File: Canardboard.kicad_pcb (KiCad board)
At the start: 4 copper layers, 50 x 58.8 mm, 149 parts, among them IC1 SIC437DED-T1-GE3, J1 RBUS, J2 USB_C_Receptacle_USB2.0, J3 Micro_SD_Card_Det, J4 Conn_01x02_Male, J5 Conn_01x03_Male, J6 Conn_01x03_Male, J7 Conn_01x03_Male, Q1 PXP012-30QLJ, Q2 PXP012-30QLJ, Q4 PXP012-30QLJ, Q6 PXP012-30QLJ, U1 ESP32-S3, U10 MP28167GQ-A-Z, U2 SN65HVD230, U3 LTC4412xS6, U4 LTC4412xS6, U7 ICM-20608-G, U8 MMC5983MA, Y1 40MHz±10ppm

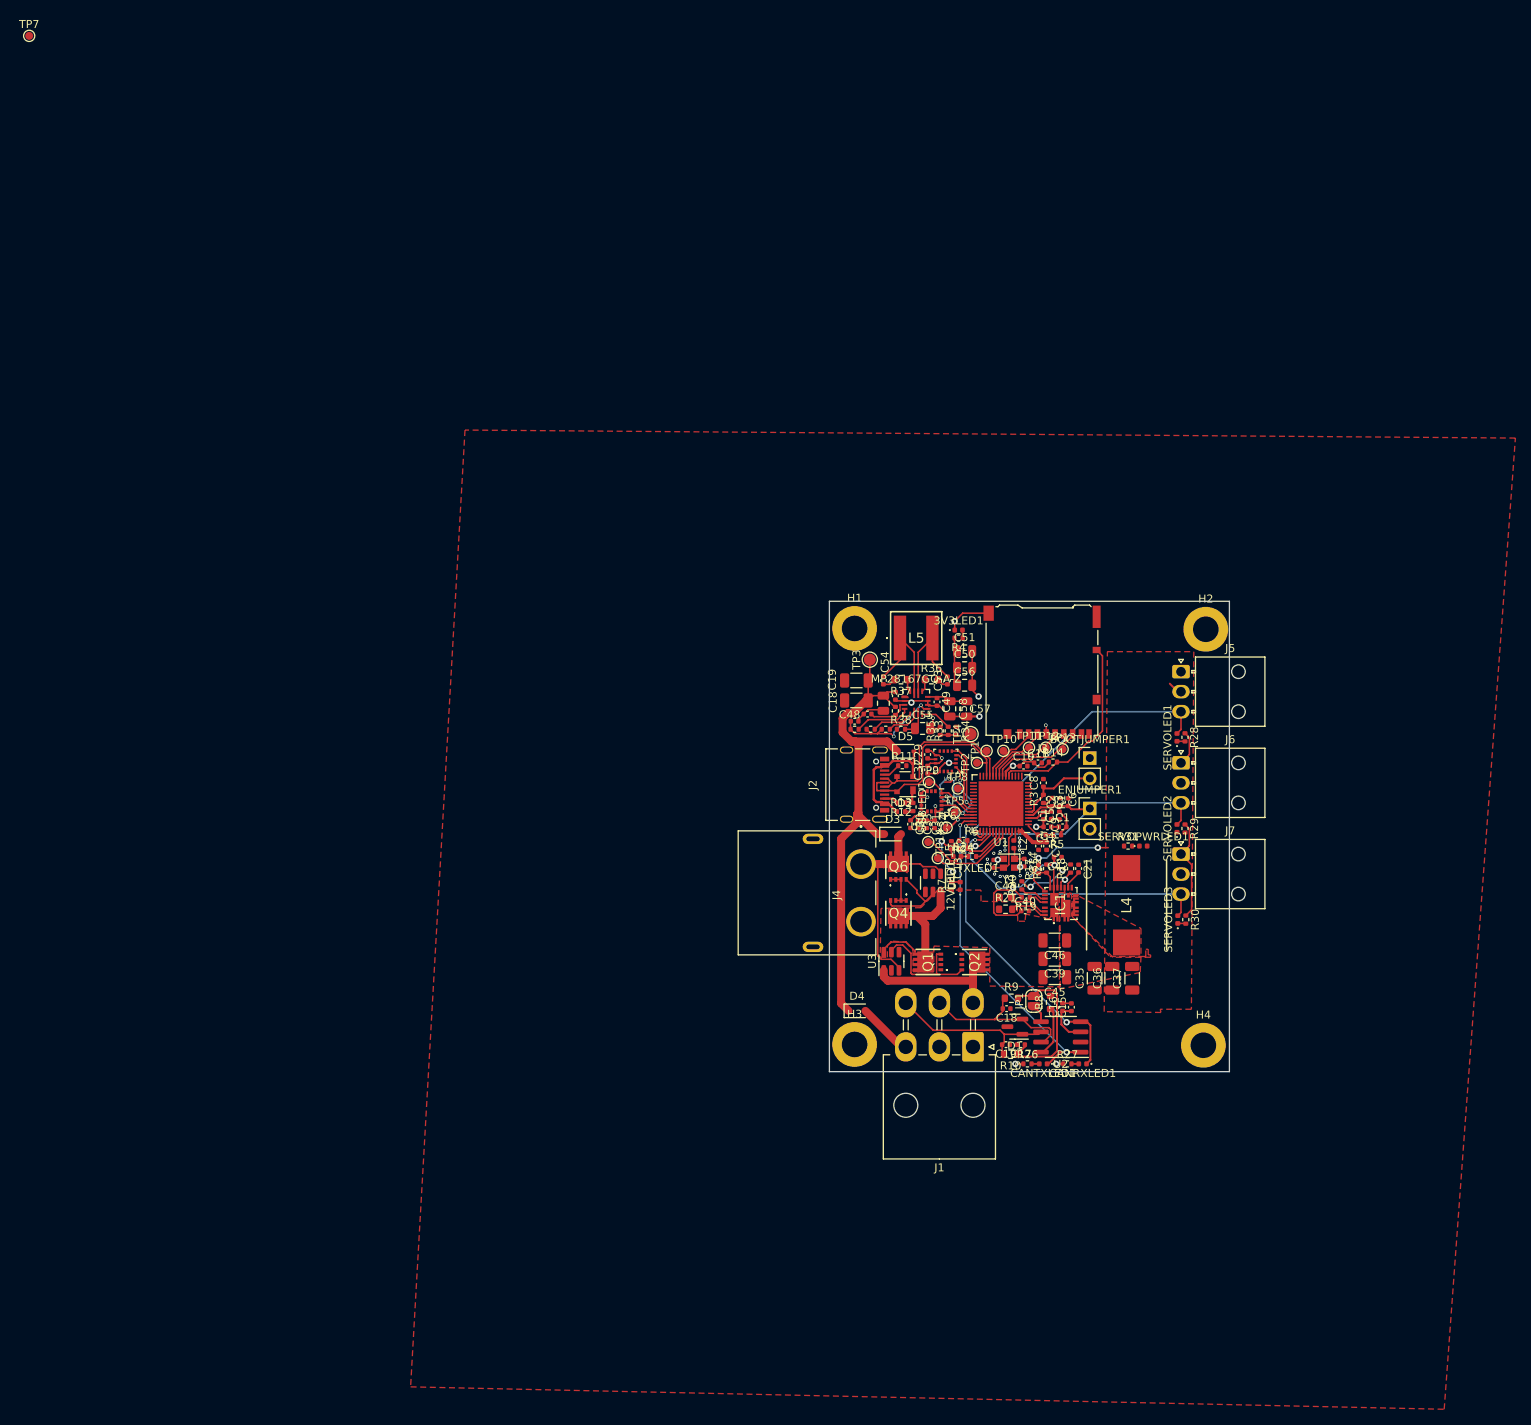
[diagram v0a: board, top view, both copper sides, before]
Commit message: weird 3v3 and 3.3v bug
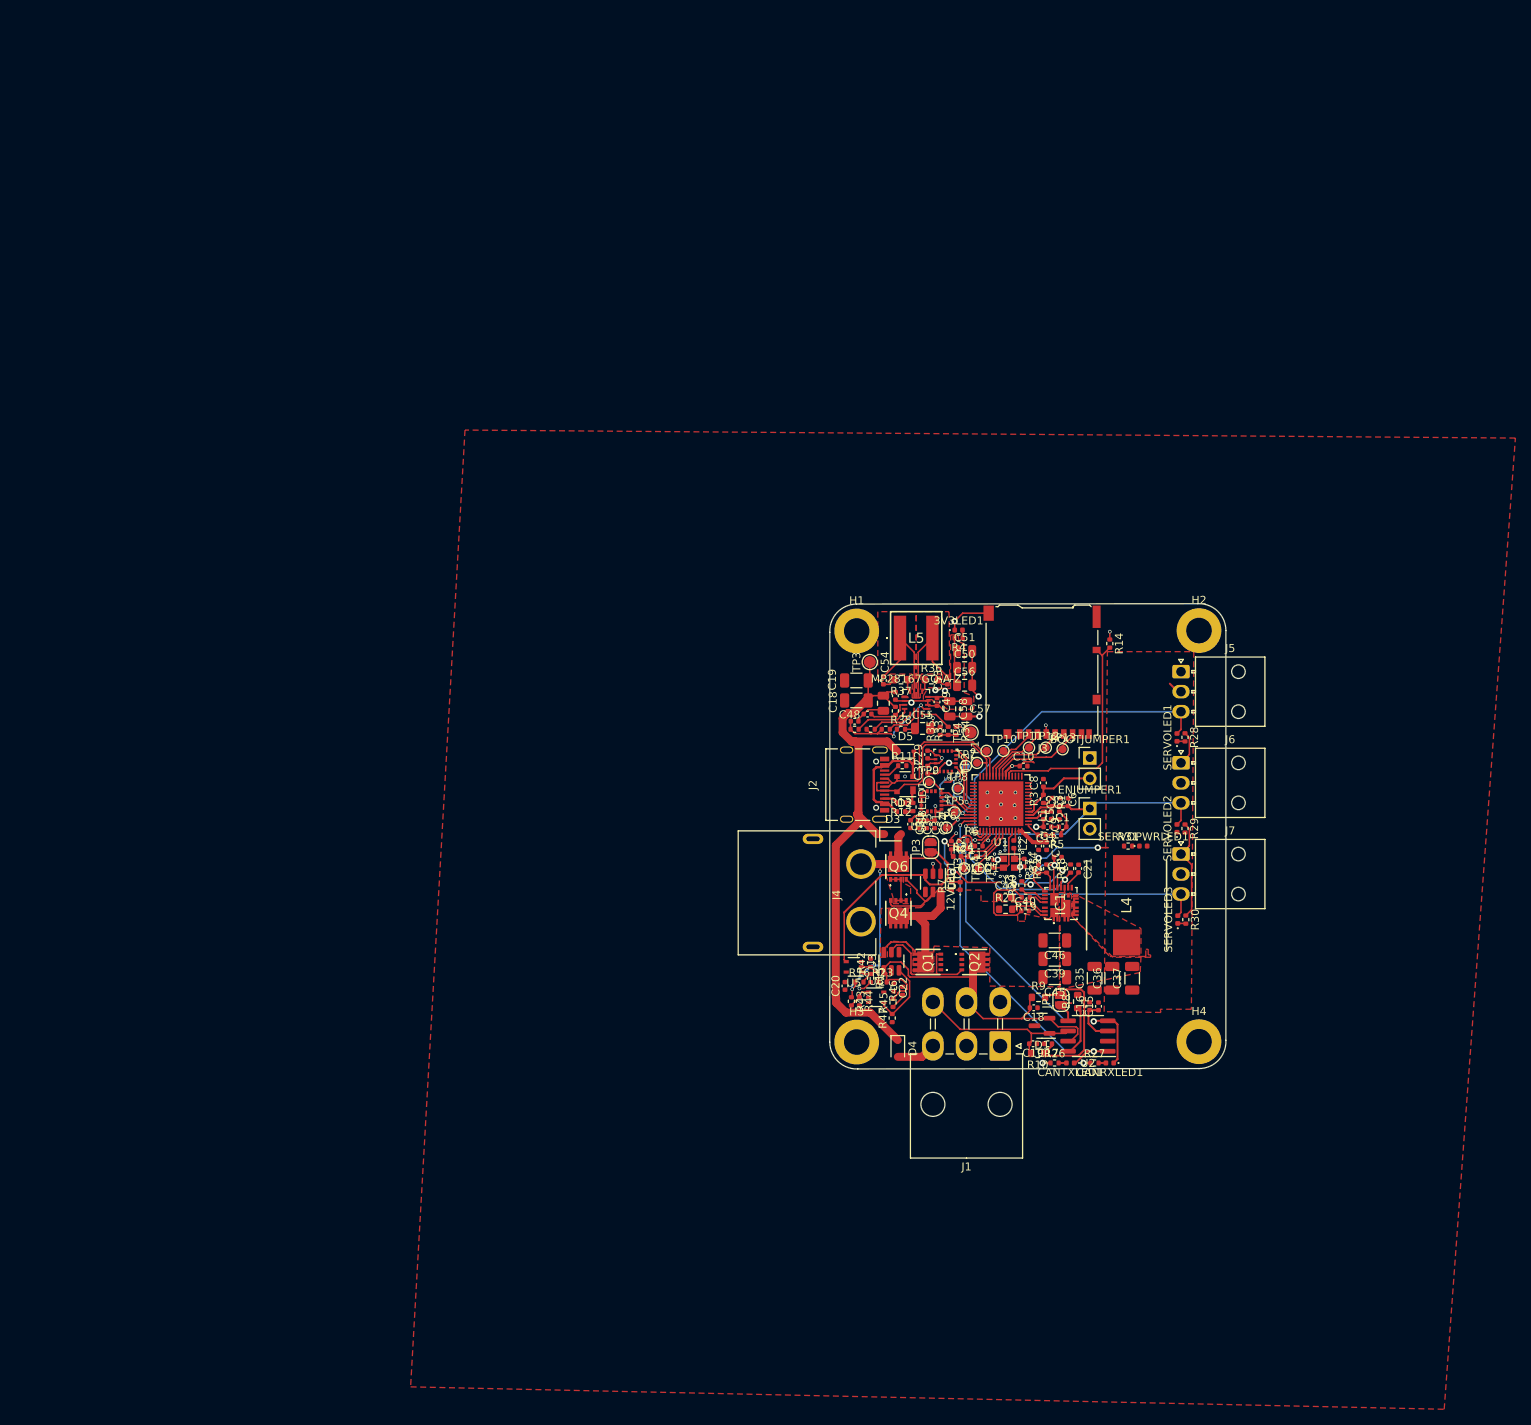
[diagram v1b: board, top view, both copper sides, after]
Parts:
- added C20: 1uF, Capacitor_SMD:C_0402_1005Metric, F.Cu at (103.0, 119.8)
- added C22: 1uF, Capacitor_SMD:C_0402_1005Metric, F.Cu at (109.1, 120.0)
- added JP3: SolderJumper_2_Open, Jumper:SolderJumper-2_P1.3mm_Open_RoundedPad1.0x1.5mm, F.Cu at (113.7, 102.5)
- added R15: 570, Resistor_SMD:R_0402_1005Metric, F.Cu at (106.2, 118.8)
- added R16: 1.5k, Resistor_SMD:R_0402_1005Metric, F.Cu at (104.8, 119.3)
- added R23: 1.5k, Resistor_SMD:R_0402_1005Metric, F.Cu at (107.7, 119.3)
- added R42: 570, Resistor_SMD:R_0402_1005Metric, F.Cu at (106.2, 116.9)
- added R43: 1.5k, Resistor_SMD:R_0402_1005Metric, F.Cu at (103.8, 121.7)
- added R44: 570, Resistor_SMD:R_0402_1005Metric, F.Cu at (104.8, 121.7)
- added R45: 1.5k, Resistor_SMD:R_0402_1005Metric, F.Cu at (109.0, 121.9)
- added R46: 570, Resistor_SMD:R_0402_1005Metric, F.Cu at (110.2, 120.4)
- added R47: 100k, Resistor_SMD:R_0402_1005Metric, F.Cu at (108.9, 123.8)
- added U5: 74AHC1G00, Package_TO_SOT_SMD:SOT-353_SC-70-5, F.Cu at (104.1, 117.4)
- added U6: 74AHC1G08, Package_TO_SOT_SMD:SOT-353_SC-70-5, F.Cu at (106.9, 121.2)
- moved TP7 148.5 mm to (118.1, 92.3)
- moved R14 16.4 mm to (136.1, 77.0), turned to -90 degrees
- moved C11 12.8 mm to (119.7, 102.3), turned to 180 degrees
- moved D4 6.94 mm to (109.6, 127.6), turned to -90 degrees
- moved TP14 5.58 mm to (117.9, 105.1)
- moved TP15 5.26 mm to (119.7, 105.1)
- moved C16 3.39 mm to (133.6, 122.3)
- moved R8 3.39 mm to (132.1, 121.7)
- moved D1 3.39 mm to (127.6, 124.8)
- moved R9 3.39 mm to (127.2, 121.2)
- moved C15 3.39 mm to (134.7, 122.3)
- moved C17 3.39 mm to (128.4, 127.0)
- moved C18 3.39 mm to (126.6, 122.5)
- moved C19 3.39 mm to (126.5, 127.0)
- moved CANRXLED1 3.39 mm to (136.1, 129.4)
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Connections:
- U3 pad 3: /rbusmosfets/BatteryPower -> Net-(U3-CTL)
- U4 pad 3: GND -> Net-(JP3-A)
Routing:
- net Net-(JP3-A): track 0.00 -> 27.2 mm
- net /servopower/PGOOD: track 9.60 -> 24.5 mm, vias 3 -> 4
- net Net-(U3-CTL): track 0.00 -> 9.30 mm
- net RBUS_uC_V: track 64.8 -> 73.5 mm
- net /rbusmosfets/RBUS_DEPL: track 17.5 -> 25.8 mm
- net GND: track 69.7 -> 74.7 mm, vias 32 -> 44
- net /rbusmosfets/BatteryPower: track 31.9 -> 36.5 mm, vias 0 -> 2
- net /RXD: track 10.8 -> 6.91 mm
- net /SERVO_SGNL1: track 35.6 -> 39.3 mm
- net /SD_DET: track 24.7 -> 28.4 mm
- net /TXD: track 6.17 -> 2.54 mm
- net Net-(R23-Pad1): track 0.00 -> 3.45 mm
- net Net-(R43-Pad2): track 0.00 -> 2.83 mm
- net Net-(R15-Pad1): track 0.00 -> 2.63 mm
- net /SPI_MISO: track 15.8 -> 18.0 mm
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- added copper zone on F.Cu, net +3V3
- added copper zone on F.Cu, net Net-(Q4-S_1)
- added copper zone on F.Cu, net Net-(U10-SW1)
- added copper zone on F.Cu, net Net-(U10-SW2)
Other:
- board size 50 x 58.8 mm -> 49.5 x 58.2 mm
